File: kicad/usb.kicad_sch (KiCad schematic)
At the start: 9 parts, among them J1 USB_C_Receptacle_USB2.0_14P, U1 USBLC6-2SC6

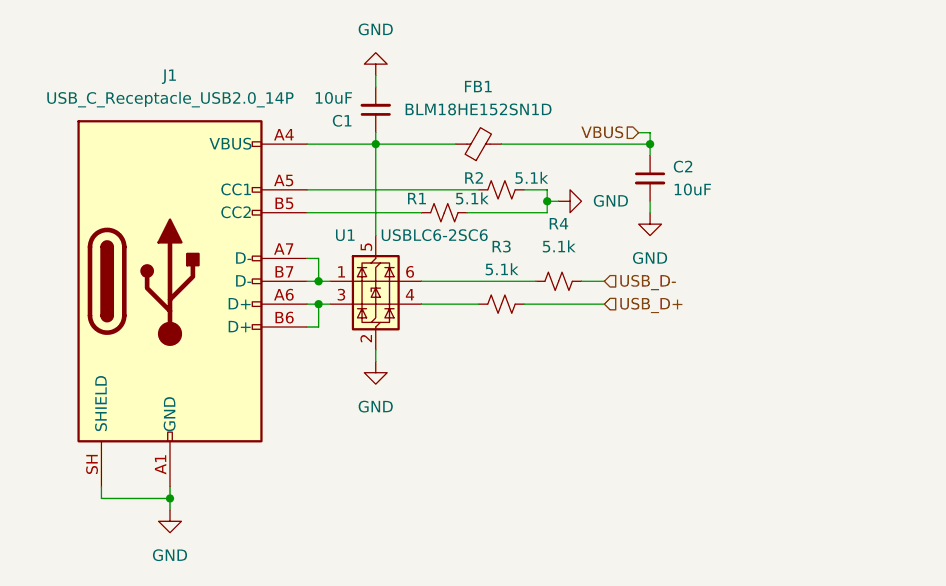
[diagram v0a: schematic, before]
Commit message: update bom and journal
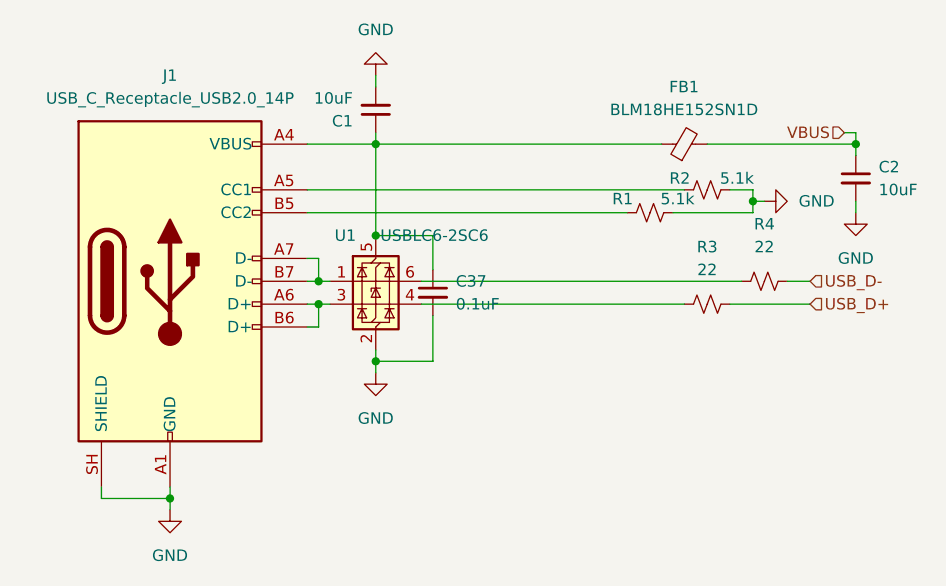
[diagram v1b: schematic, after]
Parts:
- added C37: 0.1uF, Capacitor_SMD:C_0402_1005Metric, symbol Device:C_Small
- R3, R4: value 5.1k -> 22
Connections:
- net GND: now also C37.2
- net at C1.1, FB1.1, J1.A4 (VBUS)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: now also C37.1
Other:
- moved on the sheet: C2, FB1, R1, R2, R3, R4
